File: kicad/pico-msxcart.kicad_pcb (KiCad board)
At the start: 2 copper layers, 99.7 x 62.8 mm, 15 parts, among them J1 MSX-CONNECTOR, Q1 2N3904, U1 RaspberryPi_Pico, U10 AMS1117-3.3

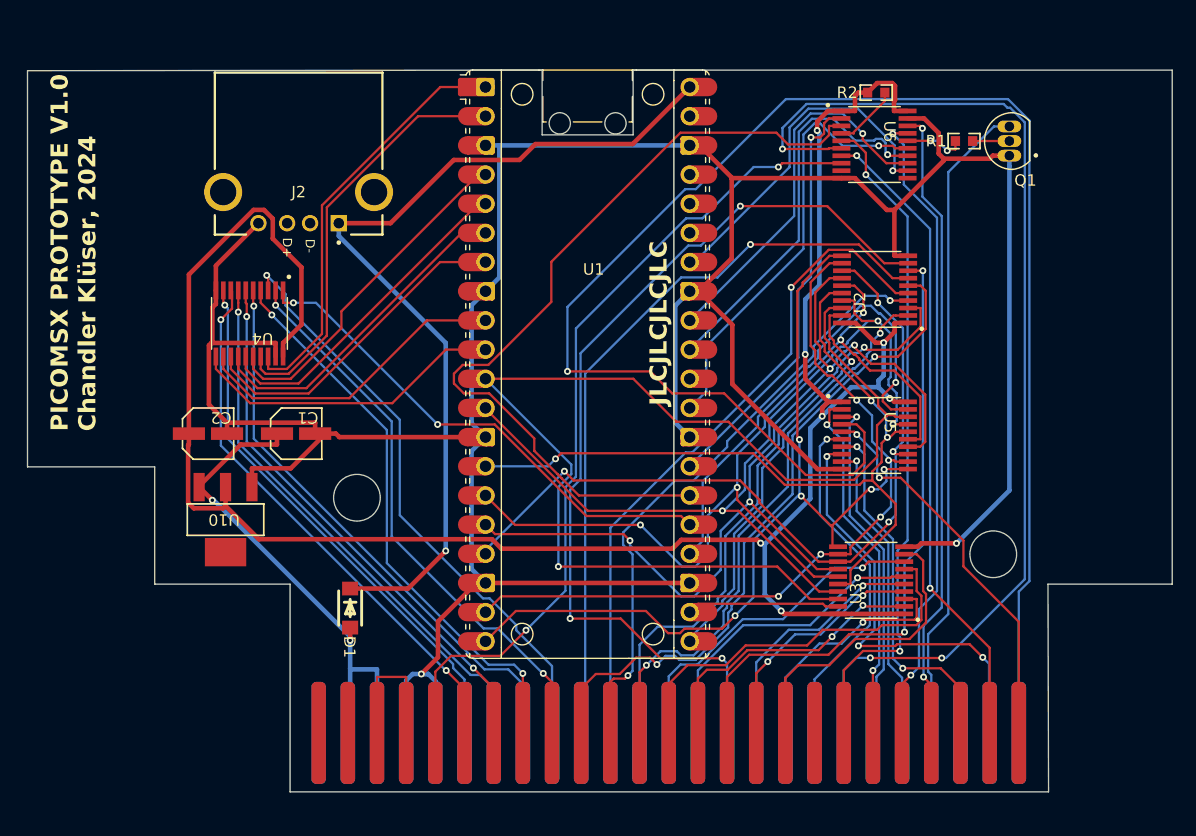
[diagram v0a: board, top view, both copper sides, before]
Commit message: Switched to Patola Board
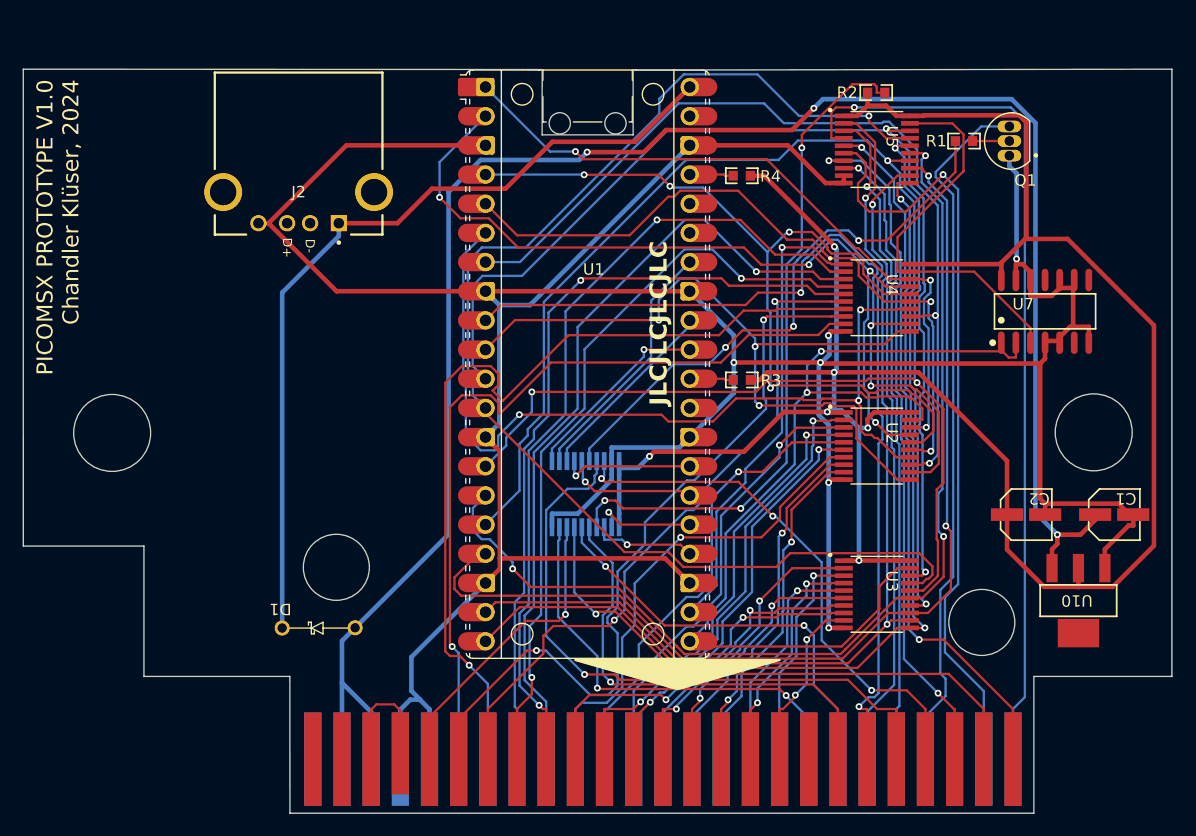
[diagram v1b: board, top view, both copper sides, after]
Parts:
- added R3: 2k2, pico-msxcart:R0603, F.Cu at (152.7, 93.0)
- added R4: 2k2, pico-msxcart:R0603, F.Cu at (152.7, 75.2)
- added U7: ~, pico-msxcart:SOP-14, F.Cu at (179.1, 87.0)
- D1: footprint pico-msxcart:SCHOTKKY -> pico-msxcart:SCHOTKKY_THT
- J1: footprint pico-msxcart:MSX-CONNECTOR2 -> pico-msxcart:MSXCART
- U6: moved to B.Cu
- moved U10 74.6 mm to (181.9, 112.0)
- moved C2 71.6 mm to (177.4, 104.7)
- moved C1 71.6 mm to (185.1, 104.7)
- moved U4 54.8 mm to (164.5, 85.9), turned to 0 degrees
- moved U6 39.5 mm to (138.9, 102.9), turned to 90 degrees
- moved U5 24.9 mm to (164.5, 73.0)
- moved U2 13.9 mm to (164.5, 98.8), turned to 0 degrees
- moved D1 4.09 mm to (115.2, 114.6), turned to 0 degrees
- moved U3 1.58 mm to (164.5, 111.8), turned to 0 degrees
- moved J1 1.29 mm to (145.8, 125.7)
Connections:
- U1 pad 1: D0_3V3 -> MP0_3V3
- U1 pad 10: D7_3V3 -> MP7_3V3
- U1 pad 11: MP0_3V3 -> MP8_3V3
- U1 pad 12: MP1_3V3 -> MP9_3V3
- U1 pad 14: MP2_3V3 -> MP10_3V3
- U1 pad 15: MP3_3V3 -> MP11_3V3
- U1 pad 16: MP4_3V3 -> MP12_3V3
- U1 pad 17: MP5_3V3 -> MP13_3V3
- U1 pad 19: MP6_3V3 -> MP14_3V3
- U1 pad 2: D1_3V3 -> MP1_3V3
- U1 pad 20: MP7_3V3 -> MP15_3V3
- U1 pad 22: MSEL1_3V3 -> DATADIR
- U1 pad 24: MSEL2_3V3 -> BUSDIR3V3
- U1 pad 25: DATADIR -> INT3V3
- U1 pad 26: BUSDIR3V3 -> RD_3V3
- U1 pad 27: INT3V3 -> WR_3V3
- U1 pad 29: RD_3V3 -> unconnected-(U1-GPIO22-Pad29)
- U1 pad 30: Net-(TP10-PROBE) -> RUN
- U1 pad 31: WR_3V3 -> RESET_3V3
- U1 pad 37: unconnected-(U1-3V3_EN-Pad37) -> 3V3_EN
- U1 pad 4: D2_3V3 -> MP2_3V3
- U1 pad 5: D3_3V3 -> MP3_3V3
- U1 pad 6: D4_3V3 -> MP4_3V3
- U1 pad 7: D5_3V3 -> MP5_3V3
- U1 pad 9: D6_3V3 -> MP6_3V3
- U3 pad 11: MP7_3V3 -> MP15_3V3
- U3 pad 12: MP6_3V3 -> MP14_3V3
- U3 pad 13: MP5_3V3 -> MP13_3V3
- U3 pad 14: MP4_3V3 -> MP12_3V3
- U3 pad 15: MP3_3V3 -> MP11_3V3
- U3 pad 16: MP2_3V3 -> MP10_3V3
- U3 pad 17: MP1_3V3 -> MP9_3V3
- U3 pad 18: MP0_3V3 -> MP8_3V3
- U3 pad 19: MSEL1_3V3 -> MSEL0_3V3
- U4 pad 11: D7_3V3 -> MP7_3V3
- U4 pad 12: D6_3V3 -> MP6_3V3
- U4 pad 13: D5_3V3 -> MP5_3V3
- U4 pad 14: D4_3V3 -> MP4_3V3
- U4 pad 15: D3_3V3 -> MP3_3V3
- U4 pad 16: D2_3V3 -> MP2_3V3
- U4 pad 17: D1_3V3 -> MP1_3V3
- U4 pad 18: D0_3V3 -> MP0_3V3
- U4 pad 19: GND -> MSEL1_3V3
- U5 pad 11: MP7_3V3 -> MP15_3V3
- U5 pad 12: MP6_3V3 -> MP14_3V3
- U5 pad 13: MP5_3V3 -> MP13_3V3
- U5 pad 14: MP4_3V3 -> MP12_3V3
- U5 pad 15: MP3_3V3 -> MP11_3V3
- U5 pad 16: MP2_3V3 -> MP10_3V3
- U5 pad 17: MP1_3V3 -> MP9_3V3
- U5 pad 18: MP0_3V3 -> MP8_3V3
- U5 pad 19: MSEL2_3V3 -> MSEL1_3V3
- U5 pad 6: RESET -> CS12
- U5 pad 8: CS12 -> M1
- U5 pad 9: M1 -> GND
- U6 pad 11: unconnected-(U6-B7-Pad11) -> RESET_3V3
- U6 pad 9: unconnected-(U6-A7-Pad9) -> RESET
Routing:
- net VCC: track 45.5 -> 160.3 mm, vias 2 -> 3
- net MP9_3V3: track 0.00 -> 110.8 mm, vias 0 -> 1
- net MP12_3V3: track 0.00 -> 101.8 mm, vias 0 -> 2
- net MP8_3V3: track 0.00 -> 94.6 mm, vias 0 -> 2
- net MP13_3V3: track 0.00 -> 91.7 mm, vias 0 -> 2
- net MP11_3V3: track 0.00 -> 91.4 mm, vias 0 -> 3
- net MP10_3V3: track 0.00 -> 86.3 mm, vias 0 -> 3
- net MP15_3V3: track 0.00 -> 84.3 mm, vias 0 -> 2
- net MP14_3V3: track 0.00 -> 82.9 mm, vias 0 -> 2
- net CS1: track 142.8 -> 76.8 mm
- net WR: track 100.8 -> 36.5 mm, vias 3 -> 2
- net BUSDIR3V3: track 72.1 -> 9.04 mm, vias 0 -> 1
- net A7: track 87.7 -> 30.2 mm, vias 3 -> 1
- net WAIT3V3: track 5.75 -> 59.1 mm, vias 0 -> 3
- net MSEL0_3V3: track 36.1 -> 85.3 mm, vias 1 -> 2
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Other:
- board size 99.7 x 62.8 mm -> 100 x 64.8 mm
